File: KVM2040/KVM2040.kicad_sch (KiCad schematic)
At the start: 2 parts, among them U1 RP2040, U2 TS3DV642A0RUAR

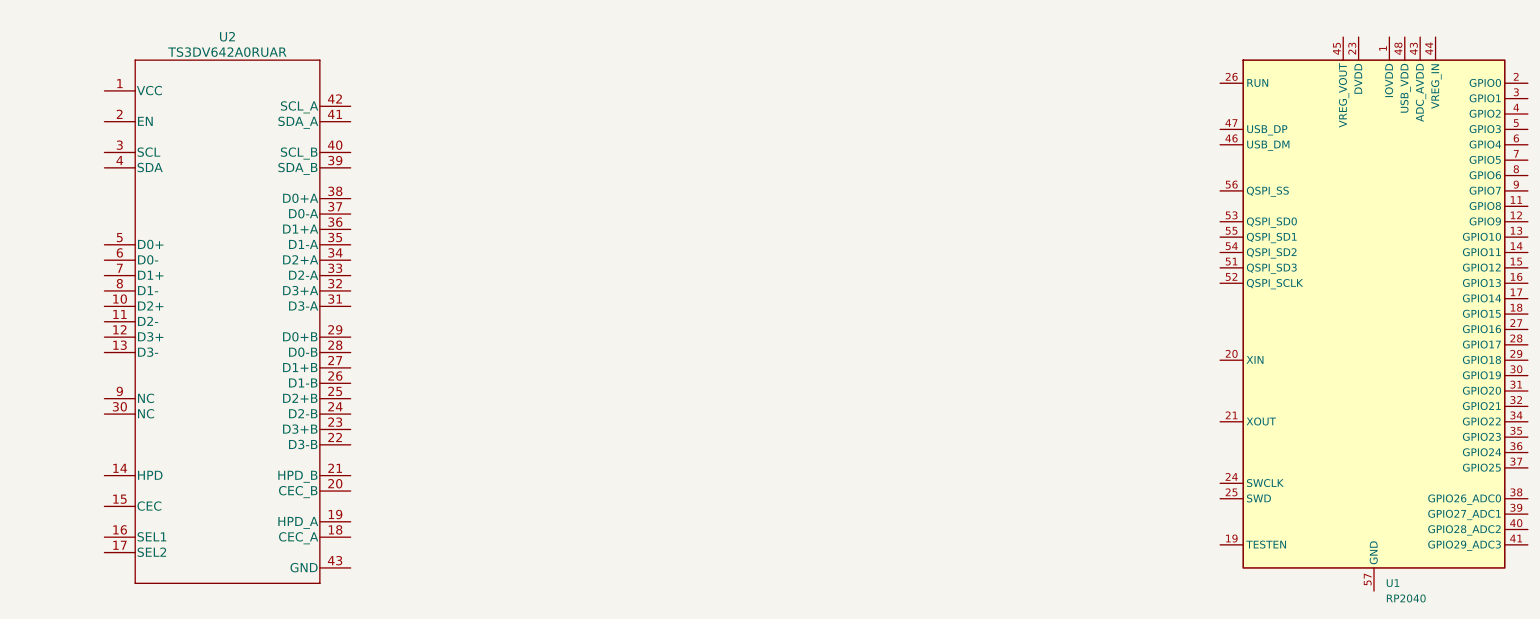
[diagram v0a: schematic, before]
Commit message: Adding some nets
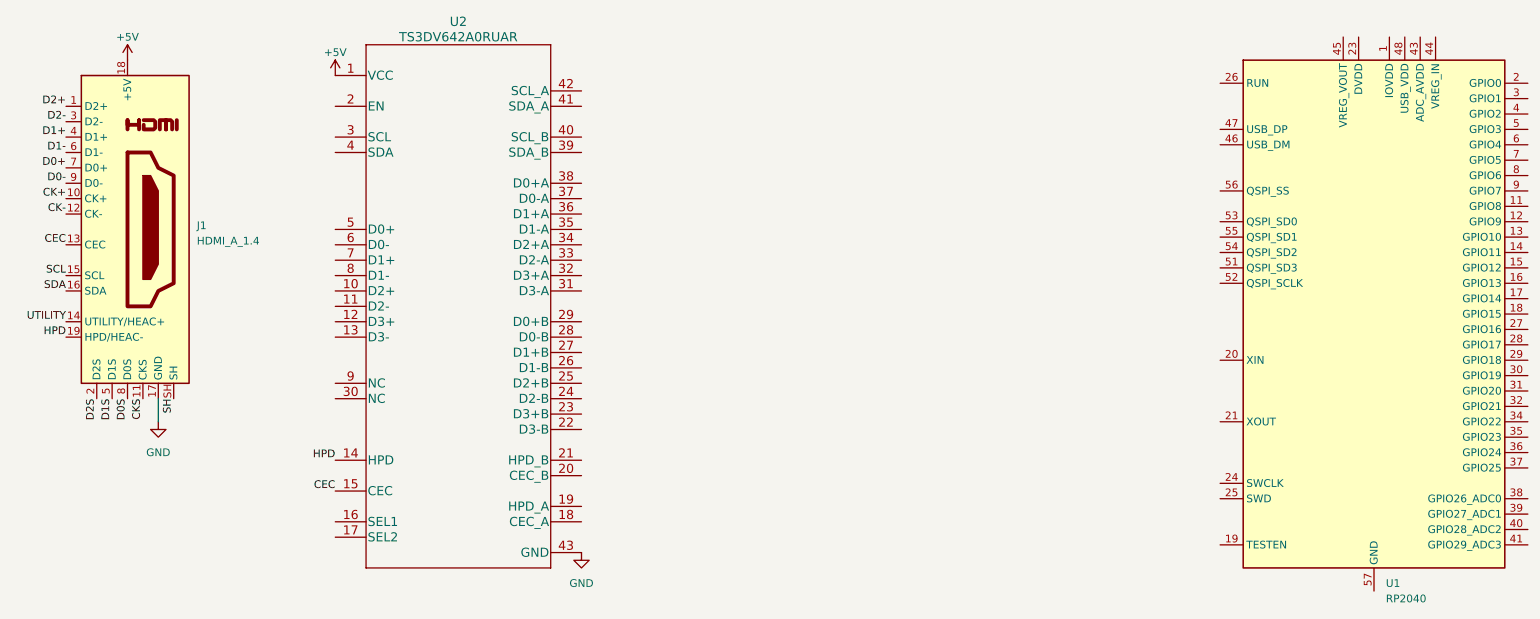
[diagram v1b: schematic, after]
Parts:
- added J1: HDMI_A_1.4, Connector_HDMI:HDMI_A_Molex_208658-1001_Horizontal, symbol Connector:HDMI_A_1.4
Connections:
- net +5V: now reaches U2.1 (VCC)
- net +5V: now also J1.18 (+5V)
- net HPD: now reaches U2.14 (HPD)
- net HPD: now also J1.19 (HPD/HEAC-)
- net CEC: now reaches U2.15 (CEC)
- net CEC: now also J1.13 (CEC)
- net GND: now reaches U2.43 (GND)
- net GND: now also J1.17 (GND)
- new net CK+: J1.10 (CK+)
- new net CK-: J1.12 (CK-)
- new net CKS: J1.11 (CKS)
- new net D0+: J1.7 (D0+)
- new net D0-: J1.9 (D0-)
- new net D0S: J1.8 (D0S)
- new net D1+: J1.4 (D1+)
- new net D1-: J1.6 (D1-)
- new net D1S: J1.5 (D1S)
- new net D2+: J1.1 (D2+)
- new net D2-: J1.3 (D2-)
- new net D2S: J1.2 (D2S)
- new net SCL: J1.15 (SCL)
- new net SDA: J1.16 (SDA)
- new net SH: J1.SH
- new net UTILITY: J1.14 (UTILITY/HEAC+)
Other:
- moved on the sheet: U2
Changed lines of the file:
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@@
 (kicad_sch (version 20230121) (generator eeschema)
   (paper "A4")
+  (wire (pts (xy 40.64 80.01) (xy 40.64 76.2))
+    (stroke (width 0) (type default))
+  )
+  (label "SH" (at 43.18 76.2 270) (fields_autoplaced)
+    (effects (font (size 1.27 1.27)) (justify right bottom))
+  )
+  (label "CEC" (at 25.4 50.8 180) (fields_autoplaced)
+    (effects (font (size 1.27 1.27)) (justify right bottom))
+  )
+  (label "D1S" (at 33.02 76.2 270) (fields_autoplaced)
+    (effects (font (size 1.27 1.27)) (justify right bottom))
+  )
+  (label "SDA" (at 25.4 58.42 180) (fields_autoplaced)
+    (effects (font (size 1.27 1.27)) (justify right bottom))
+  )
+  (label "D0+" (at 25.4 38.1 180) (fields_autoplaced)
+    (effects (font (size 1.27 1.27)) (justify right bottom))
+  )
+  (label "D0S" (at 35.56 76.2 270) (fields_autoplaced)
+    (effects (font (size 1.27 1.27)) (justify right bottom))
+  )
+  (label "SCL" (at 25.4 55.88 180) (fields_autoplaced)
+    (effects (font (size 1.27 1.27)) (justify right bottom))
+  )
+  (label "UTILITY" (at 25.4 63.5 180) (fields_autoplaced)
+    (effects (font (size 1.27 1.27)) (justify right bottom))
+  )
+  (label "D2S" (at 30.48 76.2 270) (fields_autoplaced)
+    (effects (font (size 1.27 1.27)) (justify right bottom))
+  )
+  (label "D2-" (at 25.4 30.48 180) (fields_autoplaced)
+    (effects (font (size 1.27 1.27)) (justify right bottom))
+  )
+  (label "D1-" (at 25.4 35.56 180) (fields_autoplaced)
+    (effects (font (size 1.27 1.27)) (justify right bottom))
+  )
+  (label "D0-" (at 25.4 40.64 180) (fields_autoplaced)
+    (effects (font (size 1.27 1.27)) (justify right bottom))
+  )
+  (label "HPD" (at 69.85 86.36 180) (fields_autoplaced)
+    (effects (font (size 1.27 1.27)) (justify right bottom))
+  )
+  (label "HPD" (at 25.4 66.04 180) (fields_autoplaced)
+    (effects (font (size 1.27 1.27)) (justify right bottom))
+  )
+  (label "D1+" (at 25.4 33.02 180) (fields_autoplaced)
+    (effects (font (size 1.27 1.27)) (justify right bottom))
+  )
+  (label "CEC" (at 69.85 91.44 180) (fields_autoplaced)
+    (effects (font (size 1.27 1.27)) (justify right bottom))
+  )
+  (label "CK+" (at 25.4 43.18 180) (fields_autoplaced)
+    (effects (font (size 1.27 1.27)) (justify right bottom))
+  )
+  (label "CKS" (at 38.1 76.2 270) (fields_autoplaced)
+    (effects (font (size 1.27 1.27)) (justify right bottom))
+  )
+  (label "D2+" (at 25.4 27.94 180) (fields_autoplaced)
+    (effects (font (size 1.27 1.27)) (justify right bottom))
+  )
+  (label "CK-" (at 25.4 45.72 180) (fields_autoplaced)
+    (effects (font (size 1.27 1.27)) (justify right bottom))
+  )
+  (symbol (lib_id "power:GND") (at 40.64 80.01 0) (unit 1)
+    (in_bom yes) (on_board yes) (dnp no) (fields_autoplaced)
+    (property "Reference" "#PWR01" (at 40.64 86.36 0)
+      (effects (font (size 1.27 1.27)) hide)
+    )
+    (property "Value" "GND" (at 40.64 85.09 0)
+      (effects (font (size 1.27 1.27)))
+    )
+    (property "Footprint" "" (at 40.64 80.01 0)
+      (effects (font (size 1.27 1.27)) hide)
+    )
+    (property "Datasheet" "" (at 40.64 80.01 0)
+      (effects (font (size 1.27 1.27)) hide)
+    )
+    (pin "1")
+    (instances
+      (project "KVM2040"
+        (path "/d586f62c-70f9-4a03-8772-c7cf6a61a9d8"
+          (reference "#PWR01") (unit 1)
+        )
+      )
+    )
+  )
   (symbol (lib_id "MCU_RaspberryPi:RP2040") (at 241.3 62.23 0) (unit 1)
     (in_bom yes) (on_board yes) (dnp no) (fields_autoplaced)
@@
     )
   )
-  (symbol (lib_id "TS3DV642:TS3DV642A0RUAR") (at 52.07 63.5 0) (unit 1)
-    (in_bom yes) (on_board yes) (dnp no) (fields_autoplaced)
-    (property "Reference" "U2" (at 52.07 16.51 0)
+  (symbol (lib_id "power:GND") (at 110.49 101.6 0) (unit 1)
+    (in_bom yes) (on_board yes) (dnp no) (fields_autoplaced)
+    (property "Reference" "#PWR04" (at 110.49 107.95 0)
+      (effects (font (size 1.27 1.27)) hide)
+    )
+    (property "Value" "GND" (at 110.49 106.68 0)
+      (effects (font (size 1.27 1.27)))
+    )
+    (property "Footprint" "" (at 110.49 101.6 0)
+      (effects (font (size 1.27 1.27)) hide)
+    )
+    (property "Datasheet" "" (at 110.49 101.6 0)
+      (effects (font (size 1.27 1.27)) hide)
+    )
+    (pin "1")
+    (instances
+      (project "KVM2040"
+        (path "/d586f62c-70f9-4a03-8772-c7cf6a61a9d8"
+          (reference "#PWR04") (unit 1)
+        )
+      )
+    )
+  )
+  (symbol (lib_id "power:+5V") (at 69.85 22.86 0) (unit 1)
+    (in_bom yes) (on_board yes) (dnp no) (fields_autoplaced)
+    (property "Reference" "#PWR03" (at 69.85 26.67 0)
+      (effects (font (size 1.27 1.27)) hide)
+    )
+    (property "Value" "+5V" (at 69.85 19.05 0)
+      (effects (font (size 1.27 1.27)))
+    )
+    (property "Footprint" "" (at 69.85 22.86 0)
+      (effects (font (size 1.27 1.27)) hide)
+    )
+    (property "Datasheet" "" (at 69.85 22.86 0)
+      (effects (font (size 1.27 1.27)) hide)
+    )
+    (pin "1")
+    (instances
+      (project "KVM2040"
+        (path "/d586f62c-70f9-4a03-8772-c7cf6a61a9d8"
+          (reference "#PWR03") (unit 1)
+        )
+      )
+    )
+  )
+  (symbol (lib_id "Connector:HDMI_A_1.4") (at 35.56 48.26 0) (unit 1)
+    (in_bom yes) (on_board yes) (dnp no) (fields_autoplaced)
+    (property "Reference" "J1" (at 46.99 47.625 0)
+      (effects (font (size 1.27 1.27)) (justify left))
+    )
+    (property "Value" "HDMI_A_1.4" (at 46.99 50.165 0)
+      (effects (font (size 1.27 1.27)) (justify left))
+    )
+    (property "Footprint" "Connector_HDMI:HDMI_A_Molex_208658-1001_Horizontal" (at 36.195 48.26 0)
+      (effects (font (size 1.27 1.27)) hide)
+    )
+    (property "Datasheet" "https://en.wikipedia.org/wiki/HDMI" (at 36.195 48.26 0)
+      (effects (font (size 1.27 1.27)) hide)
+    )
+    (pin "1")
+    (pin "10")
+    (pin "11")
+    (pin "12")
+    (pin "13")
+    (pin "14")
+    (pin "15")
+    (pin "16")
+    (pin "17")
+    (pin "18")
+    (pin "19")
+    (pin "2")
+    (pin "3")
+    (pin "4")
+    (pin "5")
+    (pin "6")
+    (pin "7")
+    (pin "8")
+    (pin "9")
+    (pin "SH")
+    (instances
+      (project "KVM2040"
+        (path "/d586f62c-70f9-4a03-8772-c7cf6a61a9d8"
+          (reference "J1") (unit 1)
+        )
+      )
+    )
+  )
+  (symbol (lib_id "TS3DV642:TS3DV642A0RUAR") (at 90.17 60.96 0) (unit 1)
+    (in_bom yes) (on_board yes) (dnp no) (fields_autoplaced)
+    (property "Reference" "U2" (at 90.17 13.97 0)
       (effects (font (size 1.524 1.524)))
     )
-    (property "Value" "TS3DV642A0RUAR" (at 52.07 19.05 0)
+    (property "Value" "TS3DV642A0RUAR" (at 90.17 16.51 0)
       (effects (font (size 1.524 1.524)))
     )
-    (property "Footprint" "TS3DV642:TS3DV642A0RUAR" (at 52.07 65.024 0)
+    (property "Footprint" "TS3DV642:TS3DV642A0RUAR" (at 90.17 62.484 0)
       (effects (font (size 1.524 1.524)) hide)
     )
-    (property "Datasheet" "" (at 52.07 63.5 0)
+    (property "Datasheet" "" (at 90.17 60.96 0)
       (effects (font (size 1.524 1.524)))
     )
@@
         )
       )
+    )
+  )
+  (symbol (lib_id "power:+5V") (at 35.56 20.32 0) (unit 1)
+    (in_bom yes) (on_board yes) (dnp no) (fields_autoplaced)
+    (property "Reference" "#PWR02" (at 35.56 24.13 0)
+      (effects (font (size 1.27 1.27)) hide)
+    )
+    (property "Value" "+5V" (at 35.56 16.51 0)
+      (effects (font (size 1.27 1.27)))
+    )
+    (property "Footprint" "" (at 35.56 20.32 0)
+      (effects (font (size 1.27 1.27)) hide)
+    )
+    (property "Datasheet" "" (at 35.56 20.32 0)
+      (effects (font (size 1.27 1.27)) hide)
+    )
+    (pin "1")
+    (instances
+      (project "KVM2040"
+        (path "/d586f62c-70f9-4a03-8772-c7cf6a61a9d8"
+          (reference "#PWR02") (unit 1)
+        )
+      )
